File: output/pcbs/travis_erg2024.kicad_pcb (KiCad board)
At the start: 2 copper layers, 393.3 x 146.1 mm, 380 parts, among them SW1 SW_PUSH_6mm_H4.3mm

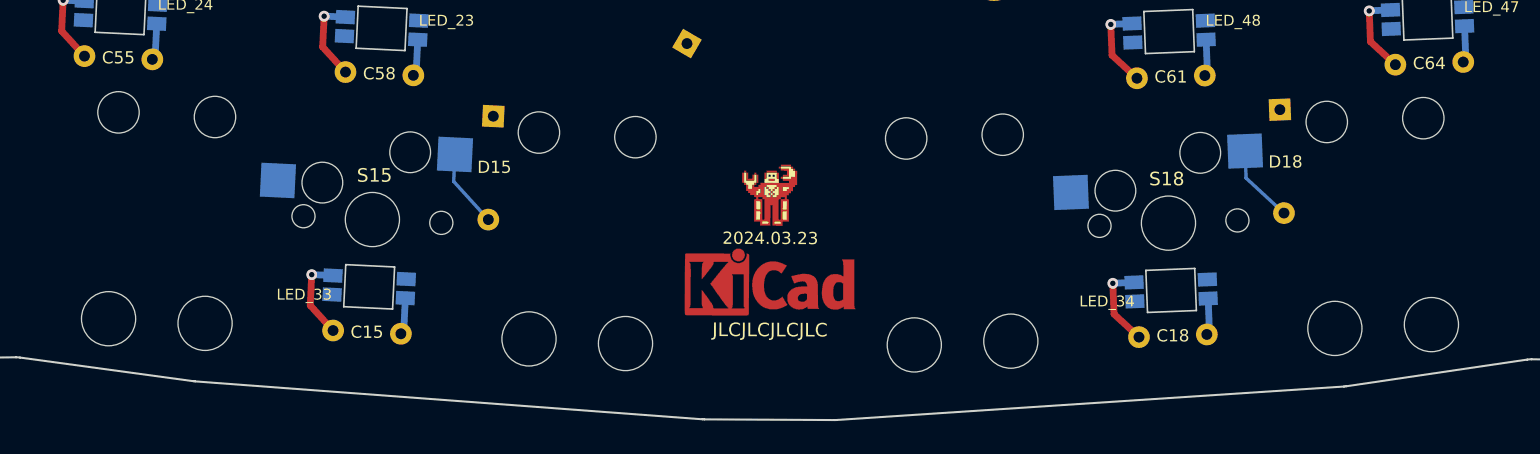
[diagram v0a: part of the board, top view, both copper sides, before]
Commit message: stab adjust
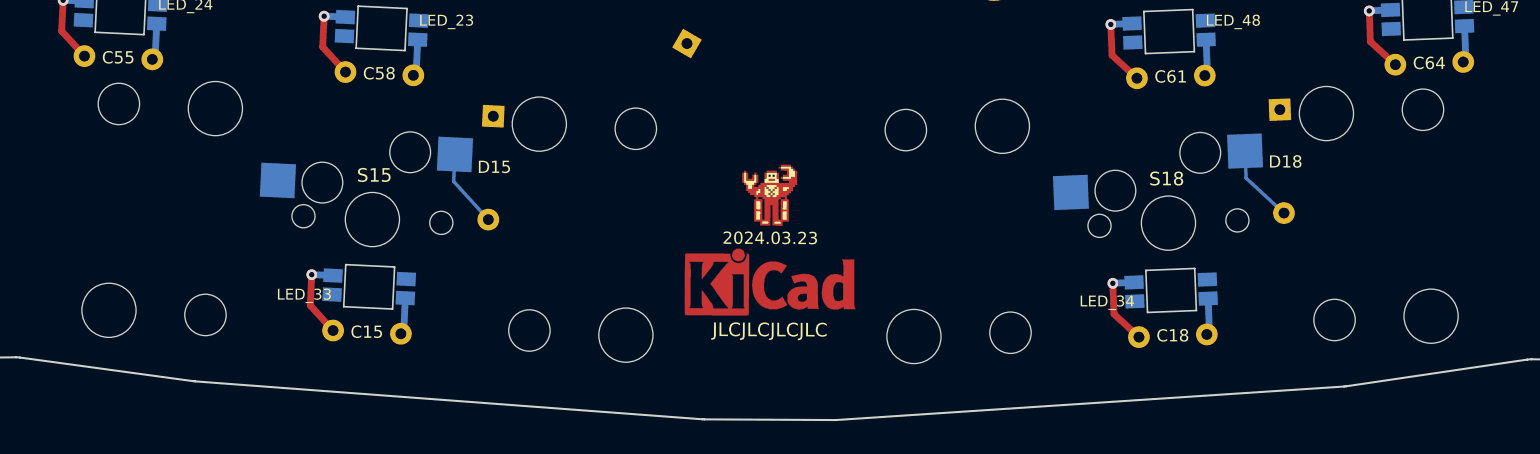
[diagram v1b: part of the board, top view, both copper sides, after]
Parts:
- moved STAB2u1 0.62 mm to (132.5, 175.3), turned to 177.25 degrees
- moved STAB3u1 0.62 mm to (132.6, 174.1)
- moved STAB2u2 0.62 mm to (191.2, 175.6), turned to 182.25 degrees
- moved STAB3u2 0.62 mm to (191.1, 174.3)
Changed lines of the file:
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@@
     (descr "MX PCB Stabilizer 2.00u 2.25u 2.50u 2.75u")
     (tags "MX Keyboard Stabilizer 2.00u 2.25u 2.50u 2.75u Cutout")
-    (at 132.5415574 174.6982491 -2.75)
+    (at 132.511811 175.3175351 177.25)
     (attr virtual)
     (fp_text reference "STAB2u1" (at 0 -2) (layer F.SilkS) hide
@@
     (descr "MX PCB Stabilizer 3.00u")
     (tags "MX Keyboard Stabilizer 3.00u Cutout")
-    (at 132.5415574 174.6982491 -2.75)
+    (at 132.57130379999998 174.0789631 -2.75)
     (attr virtual)
     (fp_text reference "STAB3u1" (at 0 -2) (layer F.SilkS) hide
@@
     (descr "MX PCB Stabilizer 2.00u 2.25u 2.50u 2.75u")
     (tags "MX Keyboard Stabilizer 2.00u 2.25u 2.50u 2.75u Cutout")
-    (at 191.1486452 174.9627056 2.25)
+    (at 191.1729863 175.58222759999998 182.25)
     (attr virtual)
     (fp_text reference "STAB2u2" (at 0 -2) (layer F.SilkS) hide
@@
     (descr "MX PCB Stabilizer 3.00u")
     (tags "MX Keyboard Stabilizer 3.00u Cutout")
-    (at 191.1486452 174.9627056 2.25)
+    (at 191.12430410000002 174.3431836 2.25)
     (attr virtual)
     (fp_text reference "STAB3u2" (at 0 -2) (layer F.SilkS) hide
